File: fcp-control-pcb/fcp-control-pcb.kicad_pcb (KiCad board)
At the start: 2 copper layers, 151.1 x 137.2 mm, 215 parts, among them IC1 L01Z050S05, J1 Conn_01x15_Female, J10 LittlePump, J11 BigPump, J12 OUT0, J13 Conn_01x10_Male, J14 Conn_01x10_Male, J15 Conn_01x10_Male, J2 Conn_01x15_Female, J3 CAPACITOR, J4 FUELCELL, J6 DISCHARGER, J7 CHARGER, J8 LimiterBypass, J9 Current_Mode, Q1 AONR21321, Q2 Q_NMOS_GDS, Q3 Q_NMOS_GDS, Q4 Q_NMOS_GDS, U1 MAX15462AB, U10 LM2902, U11 LM2902, U12 LM2902, U13 CD74HC4067SM, U14 CD74HC4067SM, U2 LM311DR, U3 TLI4971-A050T5-U-E0001, U5 LM2902, U6 LM2902, U7 LM2902, U8 LM2902, U9 LM2902

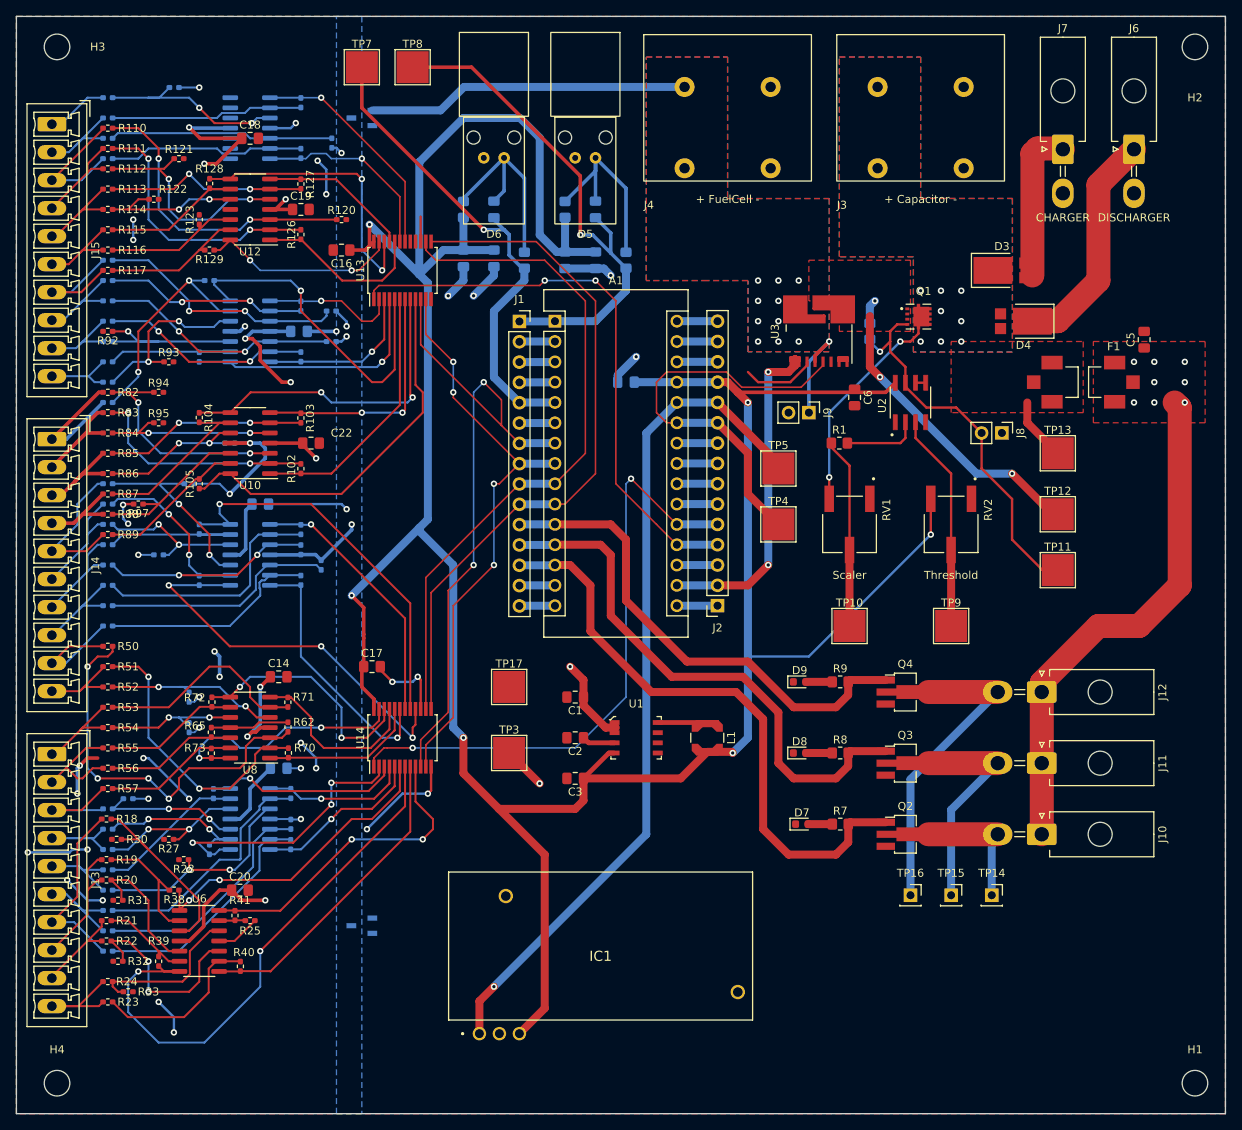
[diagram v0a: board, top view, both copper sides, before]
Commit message: layout changes
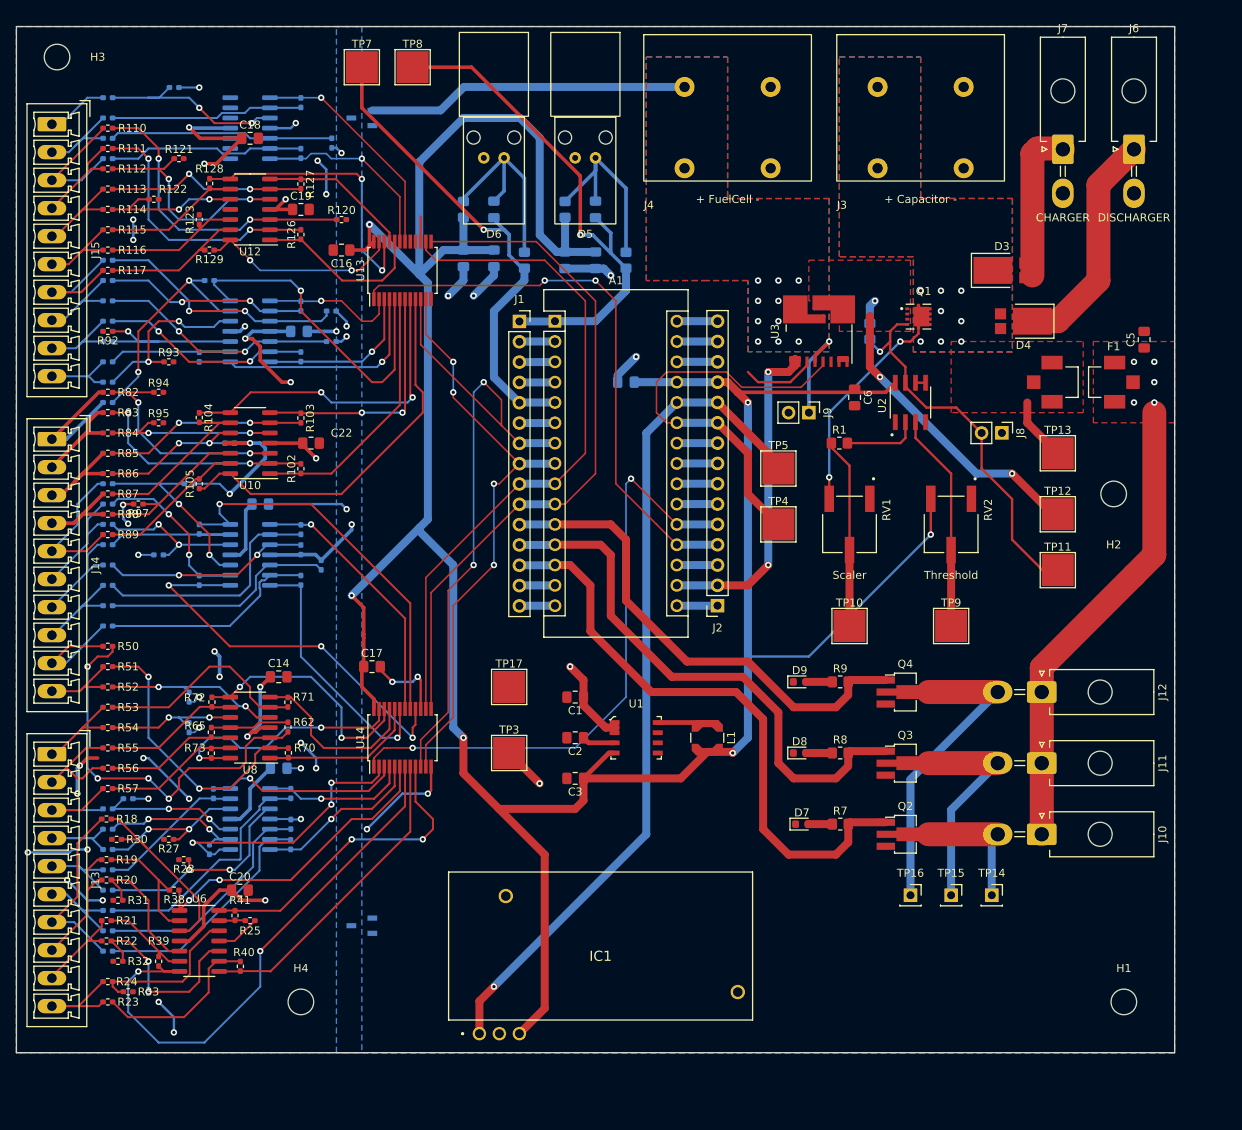
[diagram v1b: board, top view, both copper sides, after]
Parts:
- moved H2 56.8 mm to (190.5, 83.8)
- moved H4 32.1 mm to (88.9, 147.3)
- moved H1 13.5 mm to (191.8, 147.3)
- moved H3 1.27 mm to (58.4, 29.2)
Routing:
- net VCC: track 80.5 -> 74.7 mm, vias 10 -> 7
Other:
- board size 151.1 x 137.2 mm -> 144.8 x 128.3 mm
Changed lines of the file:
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@@
   )
   (footprint "MountingHole:MountingHole_3.2mm_M3" (layer "F.Cu")
-    (at 200.66 27.94)
+    (at 190.5 83.82)
     (descr "Mounting Hole 3.2mm, no annular, M3")
     (tags "mounting hole 3.2mm no annular m3")
@@
       (effects (font (size 1 1) (thickness 0.15)))
     )
-    (fp_text user "${REFERENCE}" (at 0 0) (layer "F.Fab")
-      (effects (font (size 1 1) (thickness 0.15)))
-    )
     (fp_circle (center 0 0) (end 3.2 0) (layer "Cmts.User") (width 0.15) (fill none))
     (fp_circle (center 0 0) (end 3.45 0) (layer "F.CrtYd") (width 0.05) (fill none))
@@
   )
   (footprint "MountingHole:MountingHole_3.2mm_M3" (layer "F.Cu")
-    (at 200.66 157.48)
+    (at 191.77 147.32)
     (descr "Mounting Hole 3.2mm, no annular, M3")
     (tags "mounting hole 3.2mm no annular m3")
@@
   )
   (footprint "MountingHole:MountingHole_3.2mm_M3" (layer "F.Cu")
-    (at 58.42 157.48)
+    (at 88.9 147.32)
     (descr "Mounting Hole 3.2mm, no annular, M3")
     (tags "mounting hole 3.2mm no annular m3")
@@
   )
   (footprint "MountingHole:MountingHole_3.2mm_M3" (layer "F.Cu")
-    (at 58.42 27.94)
+    (at 58.42 29.21)
     (descr "Mounting Hole 3.2mm, no annular, M3")
     (tags "mounting hole 3.2mm no annular m3")
@@
     )
   )
-  (gr_rect (start 53.34 24.13) (end 204.47 161.29) (layer "Edge.Cuts") (width 0.1) (fill none))
+  (gr_rect (start 53.34 25.4) (end 198.12 153.67) (layer "Edge.Cuts") (width 0.1) (fill none))
   (gr_text "+ FuelCell -" (at 142.24 46.99) (layer "F.SilkS")
     (effects (font (size 1 1) (thickness 0.15)))
@@
   (segment (start 106.716956 53.34) (end 109.22 53.34) (width 1) (layer "B.Cu") (net 27))
   (segment (start 135.9 67.31) (end 140.98 67.31) (width 1) (layer "B.Cu") (net 28))
-  (segment (start 188.595 100.33) (end 193.675 100.33) (width 3) (layer "F.Cu") (net 29))
-  (segment (start 181.51 107.415) (end 188.595 100.33) (width 3) (layer "F.Cu") (net 29))
+  (segment (start 181.51 108.585) (end 181.51 105.51) (width 3) (layer "F.Cu") (net 29))
   (segment (start 114.935 116.205) (end 118.745 120.015) (width 1) (layer "F.Cu") (net 29))
   (segment (start 181.51 126.365) (end 181.51 117.475) (width 3) (layer "F.Cu") (net 29))
+  (segment (start 181.51 105.51) (end 193.04 93.98) (width 3) (layer "F.Cu") (net 29))
   (segment (start 124.2275 107.0825) (end 122.555 105.41) (width 1) (layer "F.Cu") (net 29))
+  (segment (start 193.04 93.98) (end 195.58 91.44) (width 3) (layer "F.Cu") (net 29))
   (segment (start 127 113.03) (end 128.27 113.03) (width 1) (layer "F.Cu") (net 29))
-  (segment (start 181.51 108.585) (end 181.51 107.415) (width 3) (layer "F.Cu") (net 29))
   (segment (start 181.51 108.585) (end 181.51 117.475) (width 3) (layer "F.Cu") (net 29))
   (segment (start 124.2275 109.22) (end 124.2275 107.0825) (width 1) (layer "F.Cu") (net 29))
-  (segment (start 198.755 95.25) (end 198.755 73.025) (width 3) (layer "F.Cu") (net 29))
   (segment (start 124.2275 109.22) (end 124.2275 110.2575) (width 1) (layer "F.Cu") (net 29))
-  (segment (start 193.675 100.33) (end 198.755 95.25) (width 3) (layer "F.Cu") (net 29))
-  (segment (start 198.755 73.025) (end 198.12 72.39) (width 3) (layer "F.Cu") (net 29))
+  (segment (start 195.58 91.44) (end 195.58 73.66) (width 3) (layer "F.Cu") (net 29))
   (segment (start 124.2275 110.2575) (end 127 113.03) (width 1) (layer "F.Cu") (net 29))
-  (via (at 199.39 72.39) (size 0.8) (drill 0.4) (layers "F.Cu" "B.Cu") (free) (net 29))
   (via (at 193.04 67.31) (size 0.8) (drill 0.4) (layers "F.Cu" "B.Cu") (free) (net 29))
   (via (at 193.04 72.39) (size 0.8) (drill 0.4) (layers "F.Cu" "B.Cu") (free) (net 29))
   (via (at 118.745 120.015) (size 0.8) (drill 0.4) (layers "F.Cu" "B.Cu") (net 29))
-  (via (at 199.39 67.31) (size 0.8) (drill 0.4) (layers "F.Cu" "B.Cu") (free) (net 29))
   (via (at 195.58 72.39) (size 0.8) (drill 0.4) (layers "F.Cu" "B.Cu") (free) (net 29))
   (via (at 122.555 105.41) (size 0.8) (drill 0.4) (layers "F.Cu" "B.Cu") (net 29))
-  (via (at 199.39 69.85) (size 0.8) (drill 0.4) (layers "F.Cu" "B.Cu") (free) (net 29))
   (via (at 195.58 69.85) (size 0.8) (drill 0.4) (layers "F.Cu" "B.Cu") (free) (net 29))
   (via (at 195.58 67.31) (size 0.8) (drill 0.4) (layers "F.Cu" "B.Cu") (free) (net 29))
@@
     (polygon
       (pts
-        (xy 201.93 74.93)
+        (xy 198.12 74.93)
         (xy 187.96 74.93)
         (xy 187.96 64.77)
-        (xy 201.93 64.77)
+        (xy 198.12 64.77)
       )
     )
@@
     (polygon
       (pts
-        (xy 204.47 161.29)
-        (xy 53.34 161.29)
-        (xy 53.34 24.13)
-        (xy 204.47 24.13)
+        (xy 198.12 153.67)
+        (xy 53.34 153.67)
+        (xy 53.34 25.4)
+        (xy 198.12 25.4)
       )
     )
@@
     (polygon
       (pts
-        (xy 204.47 161.29)
-        (xy 93.345 161.29)
-        (xy 93.345 24.13)
-        (xy 204.47 24.13)
+        (xy 198.12 153.67)
+        (xy 93.345 153.67)
+        (xy 93.345 25.4)
+        (xy 198.12 25.4)
       )
     )
@@
     (polygon
       (pts
-        (xy 96.52 161.29)
-        (xy 53.34 161.29)
-        (xy 53.34 24.13)
-        (xy 96.52 24.13)
+        (xy 96.52 153.67)
+        (xy 53.34 153.67)
+        (xy 53.34 25.4)
+        (xy 96.52 25.4)
       )
     )
